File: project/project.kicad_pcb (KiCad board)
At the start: 2 copper layers, 67 parts, among them J1 Conn_02x16_Odd_Even, J2 TYPE-C 6P(040新), J3 Conn_01x02_Pin, SW1 SS-12D10L9, U1 DRV8833PWPR, U10 TPS22965DSGR, U11 TS5A3159ADBVR, U2 CH224K, U3 DRV8833PWPR, U4 AP63203WU, U5 TP4056, U6 AP2114, U7 MT3608L, U8 INA219AIDCNR, U9 TPS22965DSGR

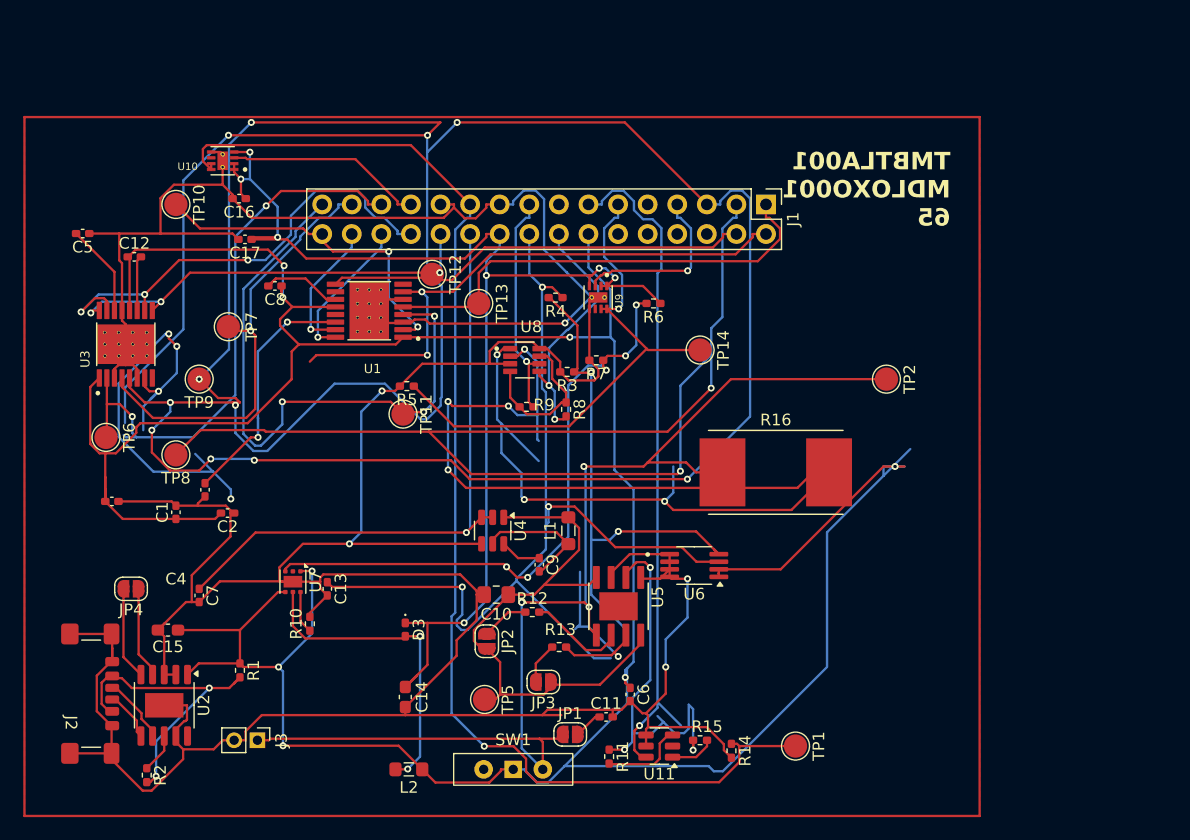
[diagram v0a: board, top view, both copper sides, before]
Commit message: Updates
Changes datasheet names,updates PCB,fixex errors
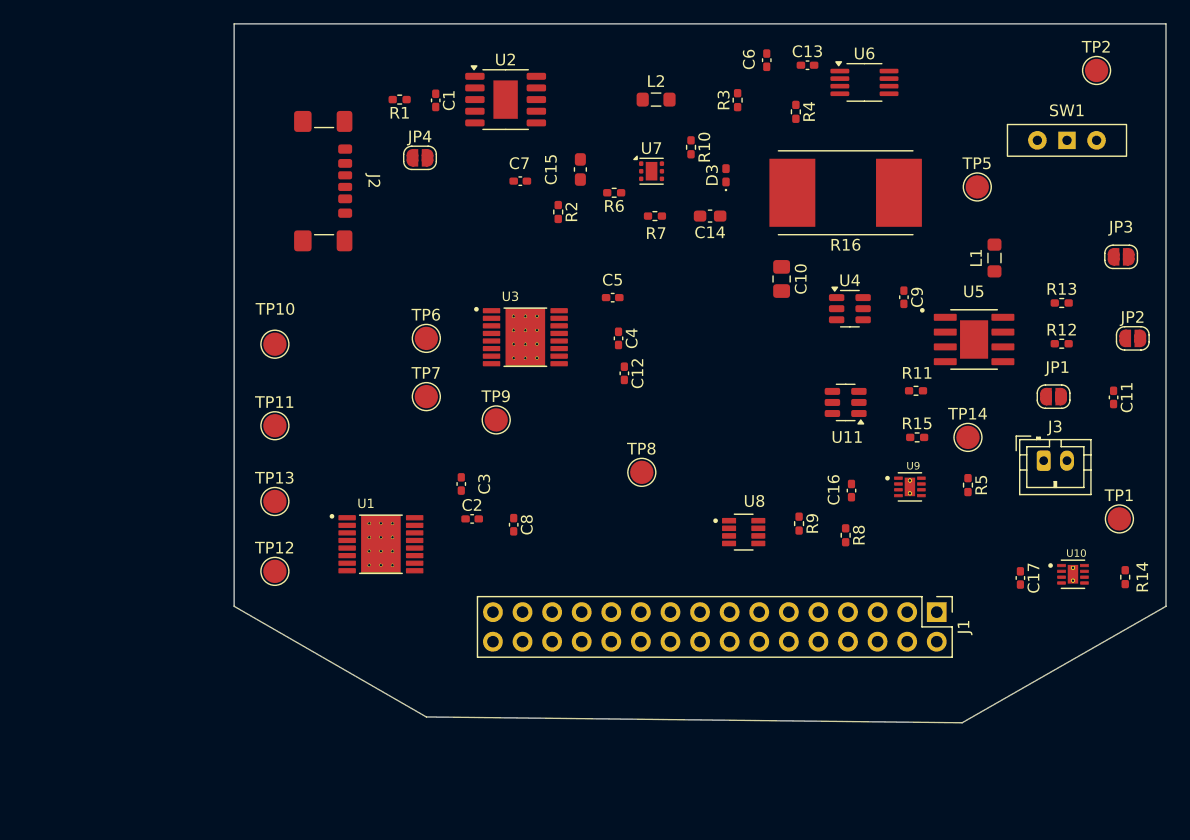
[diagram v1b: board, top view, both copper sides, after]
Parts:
- J3: footprint Connector_PinHeader_2.00mm:PinHeader_1x02_P2.00mm_Vertical -> Connector_JST:JST_PH_B2B-PH-K_1x02_P2.00mm_Vertical
- moved U10 81.2 mm to (185.5, 98.8), turned to 0 degrees
- moved C17 72.6 mm to (181.0, 99.1), turned to -90 degrees
- moved SW1 71.9 mm to (185.0, 61.5)
- moved J3 71.6 mm to (183.0, 89.0), turned to 0 degrees
- moved JP3 61.6 mm to (189.7, 71.5), turned to 0 degrees
- moved L2 61.3 mm to (149.7, 58.0), turned to 0 degrees
- moved JP2 61.2 mm to (190.7, 78.5), turned to 0 degrees
- moved TP5 61.0 mm to (177.3, 65.5), turned to 0 degrees
- moved C13 61.0 mm to (162.7, 55.0), turned to 0 degrees
- moved R2 59.9 mm to (141.3, 67.7)
- moved U2 59.7 mm to (136.8, 58.0), turned to 0 degrees
- moved C16 58.2 mm to (166.5, 91.6), turned to -90 degrees
- moved C6 55.7 mm to (159.2, 54.6)
- moved C15 53.1 mm to (143.2, 64.0), turned to -90 degrees
- moved R10 52.4 mm to (152.7, 62.1), turned to -90 degrees
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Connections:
- J1 pad 1: /Motor2_B_OUT -> /MOTOR2_B_OUT
- J1 pad 2: /Motor2_A_OUT -> /MOTOR2_A_OUT
- J1 pad 3: /Motor4_A_OUT -> /MOTOR4_A_OUT
- J1 pad 5: /Motor4_B_OUT -> /MOTOR4_B_OUT
- R8 pad 1: /3V3 -> /3V3 Out
- R9 pad 1: /3V3 -> /3V3 Out
- U3 pad 10: /MOTOR3_CTRL2 -> /MOTOR4_CTRL2
- U3 pad 9: /MOTOR3_CTRL1 -> /MOTOR4_CTRL1
- U7 pad 6: Net-(U7-OC) -> (no net)
- U8 pad 4: /3V3 -> /3V3 Out
- U8 pad 7: /3V3 -> /3V3 Out
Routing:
- net GND: track 367.5 -> 0.00 mm, vias 5 -> 0
- net /Battery: track 297.0 -> 0.00 mm, vias 8 -> 0
- net /MOTOR4_B_OUT: track 139.4 -> 0.00 mm, vias 6 -> 0
- net /Motor4_B_OUT: track 123.5 -> 0.00 mm, vias 5 -> 0
- net /EXT_LOAD1_OUT: track 107.7 -> 0.00 mm, vias 1 -> 0
- net /5V Out: track 105.8 -> 0.00 mm, vias 7 -> 0
- net /BATT: track 101.2 -> 0.00 mm, vias 3 -> 0
- net /Motor4_A_OUT: track 99.6 -> 0.00 mm, vias 1 -> 0
- net /3V3 Out: track 84.9 -> 0.00 mm, vias 3 -> 0
- net Net-(U8-IN-): track 58.9 -> 0.00 mm, vias 4 -> 0
- net /FAST_CHARGE_CTRL: track 58.6 -> 0.00 mm, vias 1 -> 0
- net /HV: track 53.5 -> 0.00 mm, vias 1 -> 0
- net /MOTOR1_B_OUT: track 53.0 -> 0.00 mm, vias 3 -> 0
- net Net-(U7-FB): track 52.4 -> 0.00 mm, vias 5 -> 0
- net Net-(U8-IN+): track 50.5 -> 0.00 mm, vias 3 -> 0
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- removed copper zone on F.Cu, net (none)
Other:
- board outline added: 80 x 60 mm
- board text removed: "TMBTLA001 MDLOXO001 65"
